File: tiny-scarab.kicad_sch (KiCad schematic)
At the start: 40 parts, among them J2 TC2050-IDC-NL, J3 CONN_PIN_HEADER_02x07, J4 CONN_PIN_HEADER_02x07, J5 3mm, J6 3mm, J7 3mm, J8 3mm

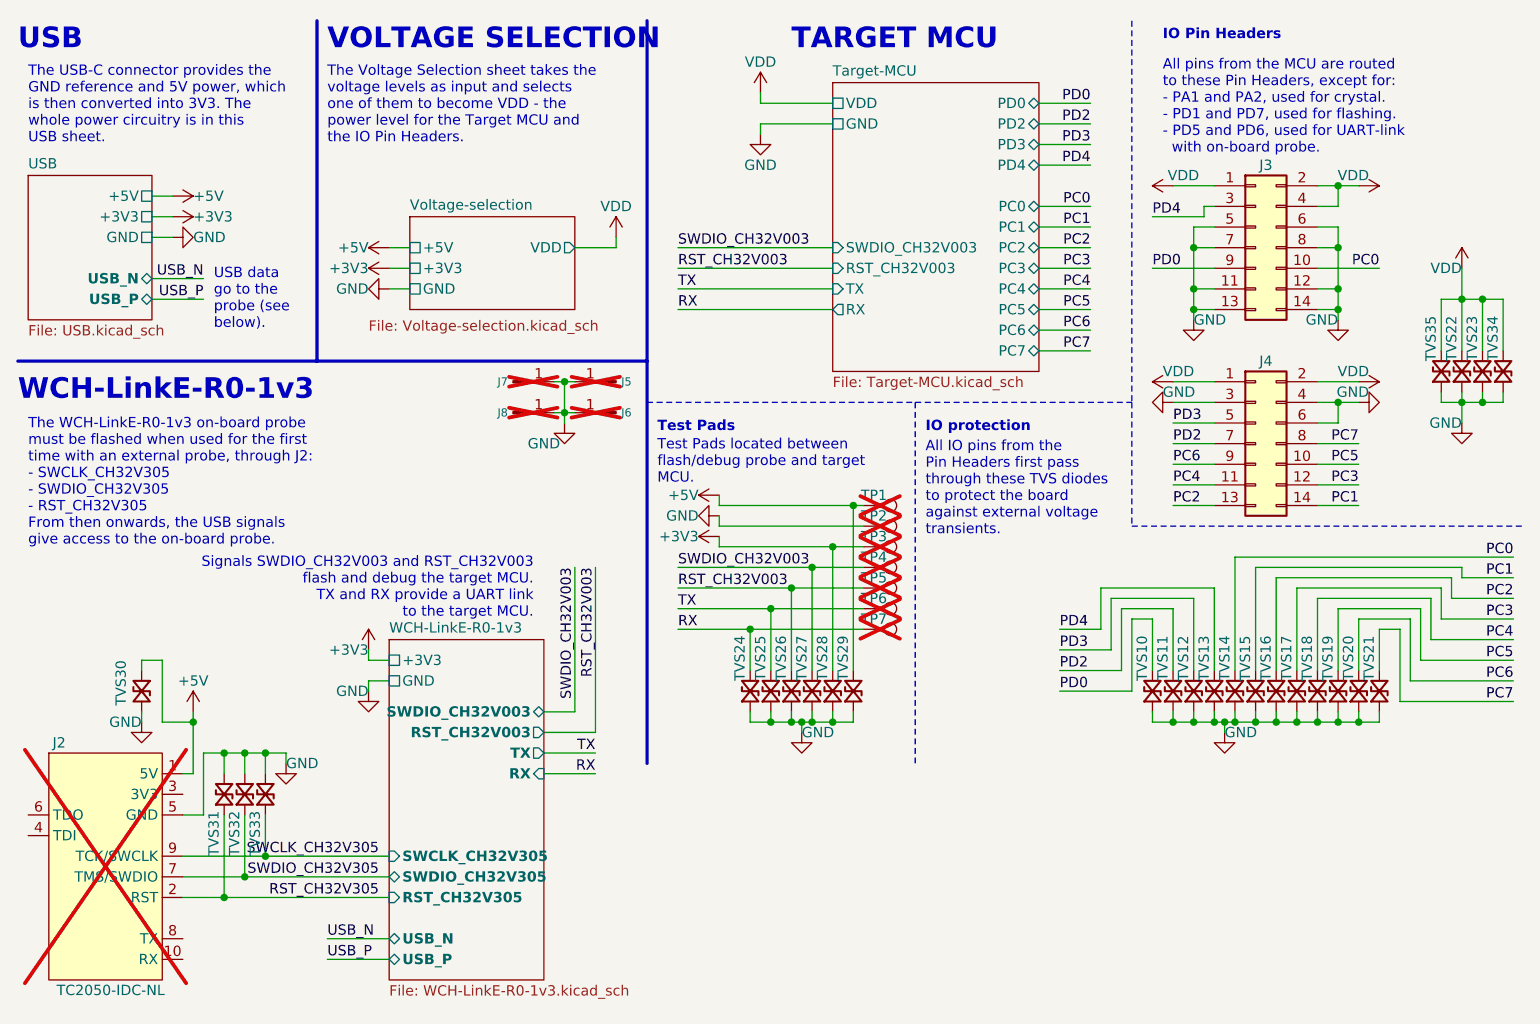
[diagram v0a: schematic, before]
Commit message: Schematic cleanup
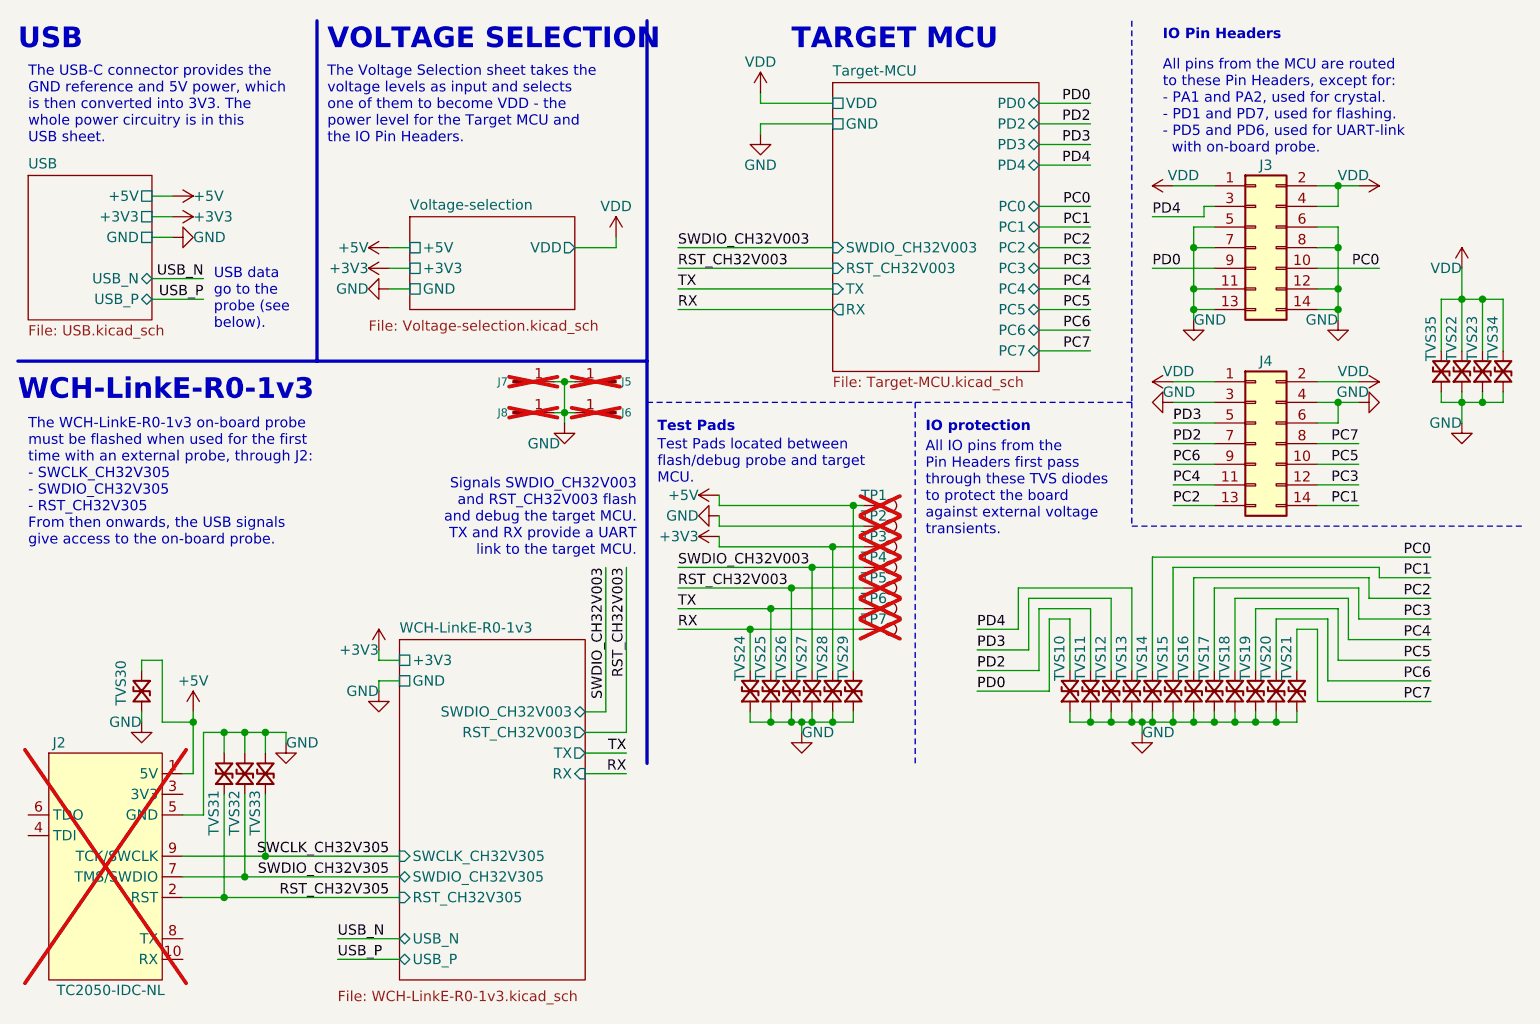
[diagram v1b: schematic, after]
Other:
- moved on the sheet: TVS10, TVS11, TVS12, TVS13, TVS14, TVS15, TVS16, TVS17, TVS18, TVS19, TVS20, TVS21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
